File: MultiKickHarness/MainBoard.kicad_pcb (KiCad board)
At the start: 2 copper layers, 83.8 x 49.5 mm, 28 parts, among them J1 Mortal Kombat 1 Y-Unit, J2 Mortal Kombat 1 T-Unit, J3 Mortal Kombat 2, J4 Mortal Kombat 3, J5 Ultimate Mortal Kombat 3, J6 Mortal Kombat 4, J6D3 P1RUN, J6D6 P2RUN, P0 MOUNTING HOLE, P1 TO CONTROL PANEL

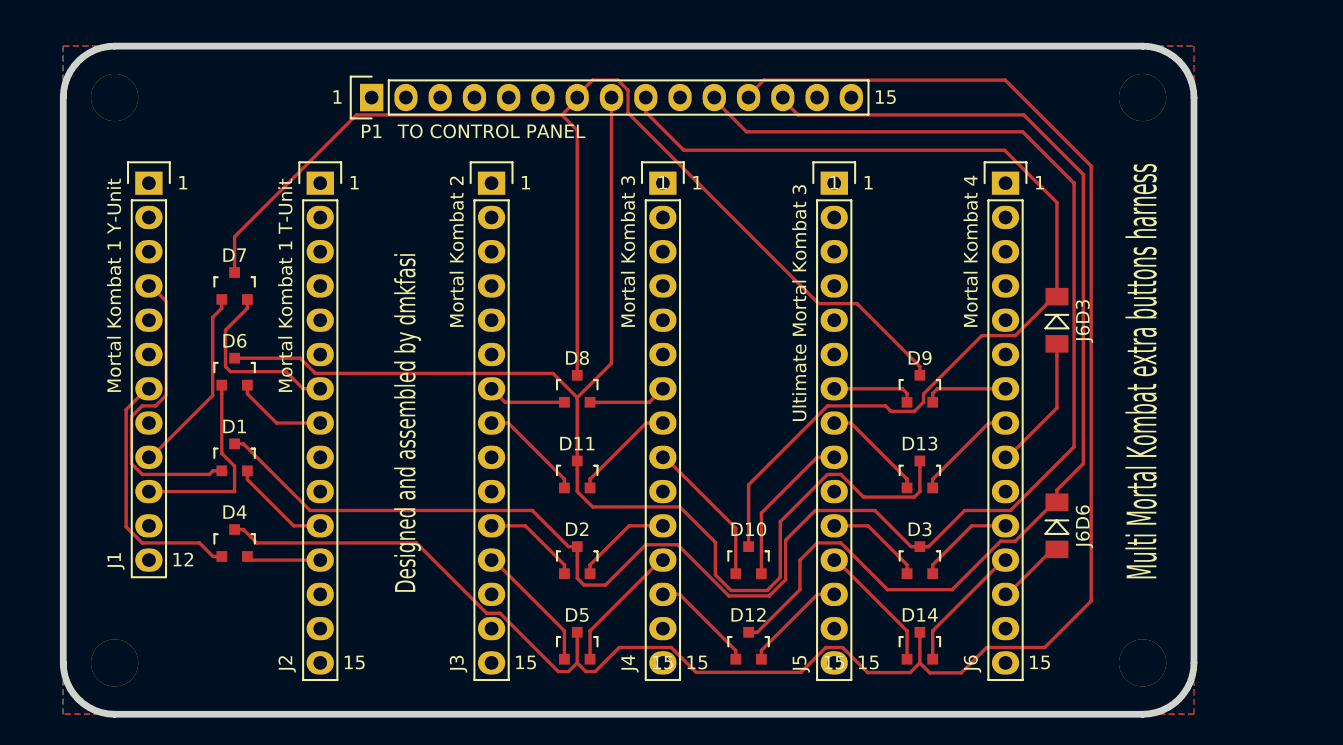
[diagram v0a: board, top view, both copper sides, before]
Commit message: New layout
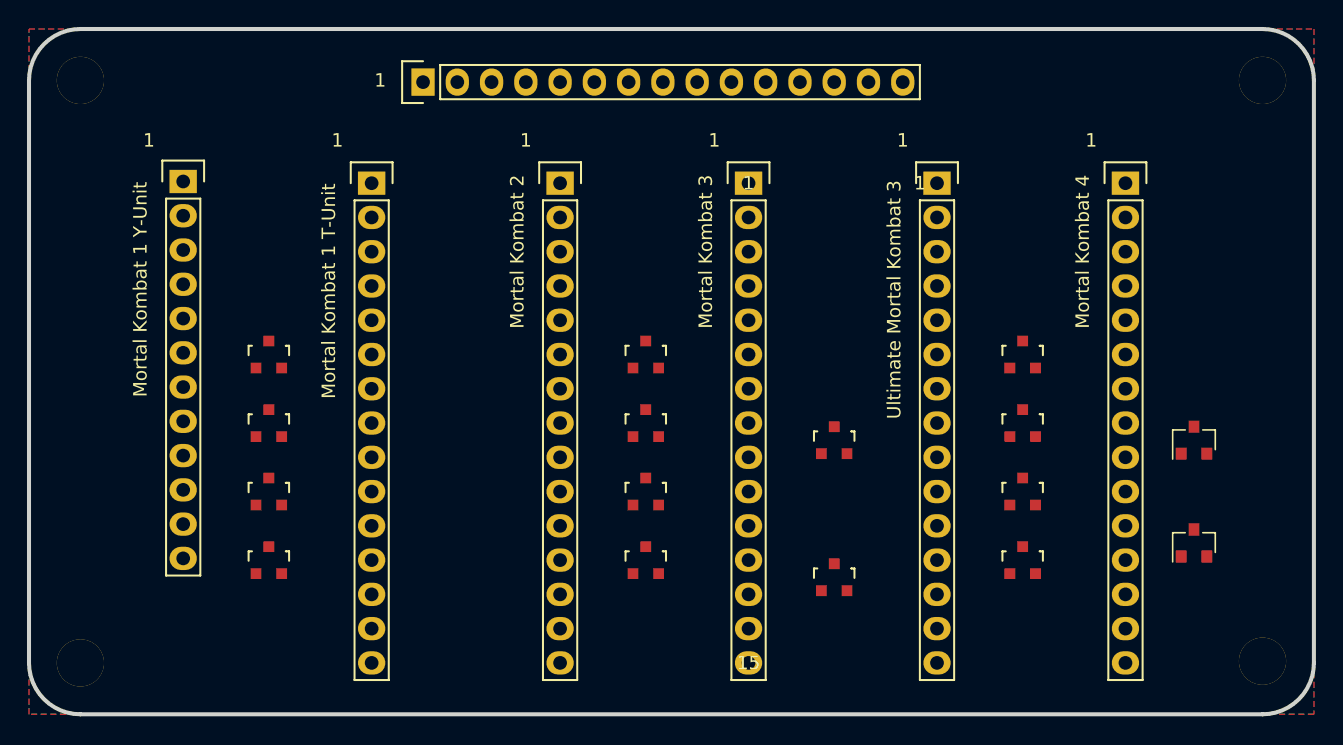
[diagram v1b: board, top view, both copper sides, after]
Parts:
- removed J6D3: P1RUN, Diodes_SMD:MiniMELF_Standard
- removed J6D6: P2RUN, Diodes_SMD:MiniMELF_Standard
- added D15: P1RUN, TO_SOT_Packages_SMD:SOT-23, F.Cu at (165.1, 127.0)
- added D16: P2RUN, TO_SOT_Packages_SMD:SOT-23, F.Cu at (165.1, 134.6)
- moved D10 10.9 mm to (138.4, 127.0)
- moved D14 9.92 mm to (152.4, 135.9)
- moved D3 9.16 mm to (152.4, 130.8)
- moved P0 8.98 mm to (170.2, 100.3)
- moved P0 8.89 mm to (170.2, 143.4)
- moved J6 8.89 mm to (160.0, 108.0)
- moved D13 8.52 mm to (152.4, 125.7)
- moved D5 8.13 mm to (124.5, 135.9)
- moved D12 8.13 mm to (138.4, 137.2)
- moved D9 8.03 mm to (152.4, 120.7)
- moved J5 7.62 mm to (146.1, 108.0)
- moved D2 7.18 mm to (124.5, 130.8)
- moved J4 6.35 mm to (132.1, 108.0)
- moved REF** 6.35 mm to (124.5, 123.2)
- moved D11 6.35 mm to (124.5, 125.7)
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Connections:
- J1 pad 11: (no net) -> Net-(J1-Pad11)
- J1 pad 12: (no net) -> Net-(J1-Pad12)
- J1 pad 2: (no net) -> Net-(J1-Pad2)
- J1 pad 3: (no net) -> Net-(J1-Pad3)
- J1 pad 5: (no net) -> Net-(J1-Pad5)
- J1 pad 6: (no net) -> Net-(J1-Pad6)
- J1 pad 8: (no net) -> Net-(J1-Pad8)
- J2 pad 10: (no net) -> Net-(J2-Pad10)
- J2 pad 13: (no net) -> Net-(J2-Pad13)
- J2 pad 14: (no net) -> Net-(J2-Pad14)
- J2 pad 15: (no net) -> Net-(J2-Pad15)
- J2 pad 2: (no net) -> Net-(J2-Pad2)
- J2 pad 3: (no net) -> Net-(J2-Pad3)
- J2 pad 4: (no net) -> Net-(J2-Pad4)
- J2 pad 5: (no net) -> Net-(J2-Pad5)
- J2 pad 6: (no net) -> Net-(J2-Pad6)
- J2 pad 9: (no net) -> Net-(J2-Pad9)
- J3 pad 10: (no net) -> Net-(J3-Pad10)
- J3 pad 13: (no net) -> Net-(J3-Pad13)
- J3 pad 14: (no net) -> Net-(J3-Pad14)
- J3 pad 15: (no net) -> Net-(J3-Pad15)
- J3 pad 2: (no net) -> Net-(J3-Pad2)
- J3 pad 3: (no net) -> Net-(J3-Pad3)
- J3 pad 4: (no net) -> Net-(J3-Pad4)
- J3 pad 5: (no net) -> Net-(J3-Pad5)
- J3 pad 6: (no net) -> Net-(J3-Pad6)
- J3 pad 9: (no net) -> Net-(J3-Pad9)
- J4 pad 10: (no net) -> Net-(J4-Pad10)
- J4 pad 14: (no net) -> Net-(J4-Pad14)
- J4 pad 15: (no net) -> Net-(J4-Pad15)
- J4 pad 2: (no net) -> Net-(J4-Pad2)
- J4 pad 3: (no net) -> Net-(J4-Pad3)
- J4 pad 4: (no net) -> Net-(J4-Pad4)
- J4 pad 5: (no net) -> Net-(J4-Pad5)
- J4 pad 6: (no net) -> Net-(J4-Pad6)
- J5 pad 10: (no net) -> Net-(J5-Pad10)
- J5 pad 14: (no net) -> Net-(J5-Pad14)
- J5 pad 15: (no net) -> Net-(J5-Pad15)
- J5 pad 2: (no net) -> Net-(J5-Pad2)
- J5 pad 3: (no net) -> Net-(J5-Pad3)
- J5 pad 4: (no net) -> Net-(J5-Pad4)
- J5 pad 5: (no net) -> Net-(J5-Pad5)
- J5 pad 6: (no net) -> Net-(J5-Pad6)
- J6 pad 10: (no net) -> Net-(J6-Pad10)
- J6 pad 14: (no net) -> Net-(J6-Pad14)
- J6 pad 15: (no net) -> Net-(J6-Pad15)
- J6 pad 2: (no net) -> Net-(J6-Pad2)
- J6 pad 3: (no net) -> Net-(J6-Pad3)
- J6 pad 4: (no net) -> Net-(J6-Pad4)
- J6 pad 5: (no net) -> Net-(J6-Pad5)
- J6 pad 6: (no net) -> Net-(J6-Pad6)
- P1 pad 10: (no net) -> Net-(P1-Pad10)
- P1 pad 14: (no net) -> Net-(P1-Pad14)
- P1 pad 15: (no net) -> Net-(P1-Pad15)
- P1 pad 2: (no net) -> Net-(P1-Pad2)
- P1 pad 3: (no net) -> Net-(P1-Pad3)
- P1 pad 4: (no net) -> Net-(P1-Pad4)
- P1 pad 5: (no net) -> Net-(P1-Pad5)
- P1 pad 6: (no net) -> Net-(P1-Pad6)
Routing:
- net /P2-LK: track 139.7 -> 0.00 mm
- net /P2-LP: track 128.2 -> 0.00 mm
- net /P1-LK: track 95.8 -> 0.00 mm
- net /P1-LP: track 88.6 -> 0.00 mm
- net /P2-RUN: track 80.8 -> 0.00 mm
- net /P1-RUN: track 75.2 -> 0.00 mm
- net Net-(D1-Pad1): track 22.6 -> 0.00 mm
- net Net-(D4-Pad1): track 19.0 -> 0.00 mm
- net Net-(D6-Pad1): track 14.6 -> 0.00 mm
- net Net-(D7-Pad1): track 14.0 -> 0.00 mm
- net Net-(D7-Pad2): track 13.4 -> 0.00 mm
- net Net-(D10-Pad2): track 11.6 -> 0.00 mm
- net Net-(D10-Pad1): track 10.9 -> 0.00 mm
- net Net-(D15-Pad1): track 10.1 -> 0.00 mm
- net Net-(D5-Pad2): track 9.68 -> 0.00 mm
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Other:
- board size 83.8 x 49.5 mm -> 95.3 x 50.8 mm
- net class Default: clearance 0.15 -> 0.2
- rule trace_clearance: 0.15 -> 0.2
- board text added: "Rev.2.1"
- board text removed: "12"
- board text removed: "Rev.2"
